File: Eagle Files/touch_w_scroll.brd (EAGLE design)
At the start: 14 x 73 mm, 3 parts

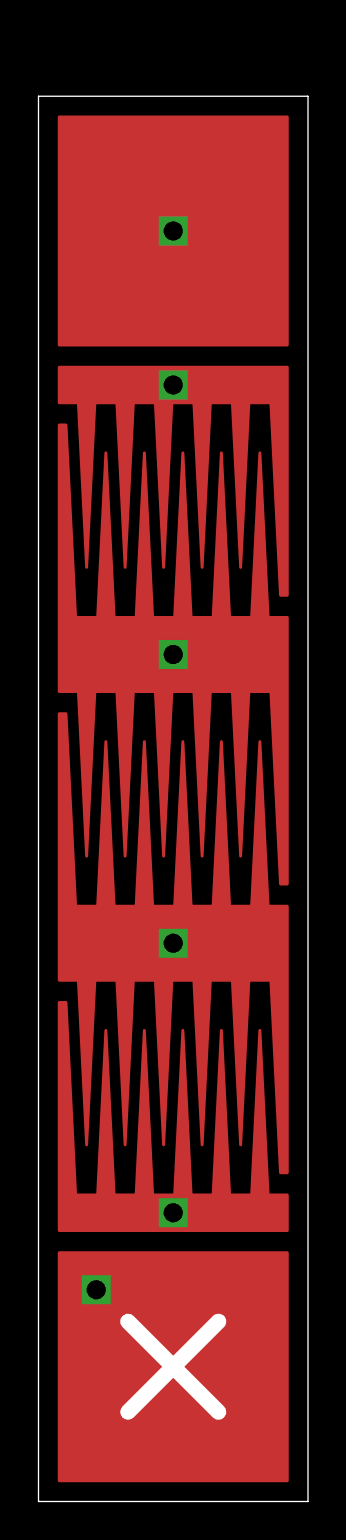
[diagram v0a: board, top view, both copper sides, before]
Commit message: maybe final touch board
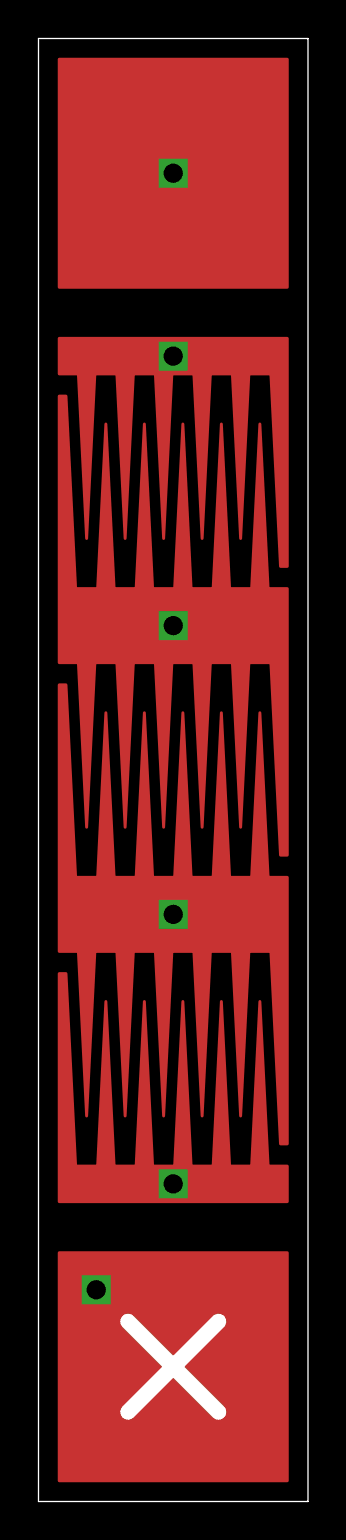
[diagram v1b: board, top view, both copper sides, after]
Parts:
- moved U$2 3.00 mm to (1.00, 75.0)
- moved U$1 1.50 mm to (13.0, 60.5)
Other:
- board size 14 x 73 mm -> 14 x 76 mm
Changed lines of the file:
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@@
 <layer number="44" name="Drills" color="7" fill="1" visible="no" active="yes"/>
 <layer number="45" name="Holes" color="7" fill="1" visible="no" active="yes"/>
-<layer number="46" name="Milling" color="3" fill="1" visible="no" active="yes"/>
+<layer number="46" name="Milling" color="3" fill="1" visible="yes" active="yes"/>
 <layer number="47" name="Measures" color="7" fill="1" visible="no" active="yes"/>
 <layer number="48" name="Document" color="7" fill="1" visible="yes" active="yes"/>
@@
 <plain>
 <wire x1="0" y1="0" x2="14" y2="0" width="0" layer="20"/>
-<wire x1="14" y1="0" x2="14" y2="73" width="0" layer="20"/>
-<wire x1="14" y1="73" x2="0" y2="73" width="0" layer="20"/>
-<wire x1="0" y1="73" x2="0" y2="0" width="0" layer="20"/>
-<wire x1="4.65" y1="9.35" x2="9.35" y2="4.65" width="0.8128" layer="20"/>
-<wire x1="4.65" y1="4.65" x2="9.35" y2="9.35" width="0.8128" layer="20"/>
+<wire x1="14" y1="0" x2="14" y2="76" width="0" layer="20"/>
+<wire x1="14" y1="76" x2="0" y2="76" width="0" layer="20"/>
+<wire x1="0" y1="76" x2="0" y2="0" width="0" layer="20"/>
 </plain>
 <attributes>
@@
 </autorouter>
 <elements>
-<element name="U$1" library="Cap Touch Pads" library_urn="urn:adsk.eagle:library:35100943" package="SLIDE" package3d_urn="urn:adsk.eagle:package:35100947/4" value="SLIDE_PAD" x="13" y="59" smashed="yes" rot="R270"/>
-<element name="U$2" library="Cap Touch Pads" library_urn="urn:adsk.eagle:library:35100943" package="12X12_PAD" package3d_urn="urn:adsk.eagle:package:35100948/2" value="12X12_PAD" x="1" y="72" smashed="yes"/>
-<element name="U$4" library="Cap Touch Pads" library_urn="urn:adsk.eagle:library:35100943" package="12X12_PAD_LED" package3d_urn="urn:adsk.eagle:package:35129608/1" value="12X12_PADLED" x="1" y="13" smashed="yes"/>
+<element name="U$1" library="Cap Touch Pads" library_urn="urn:adsk.eagle:library:35100943" package="SLIDE" package3d_urn="urn:adsk.eagle:package:35100947/4" value="SLIDE_PAD" x="13" y="60.5" smashed="yes" rot="R270"/>
+<element name="U$2" library="Cap Touch Pads" library_urn="urn:adsk.eagle:library:35100943" package="12X12_PAD" package3d_urn="urn:adsk.eagle:package:35100948/2" value="12X12_PAD" x="1" y="75" smashed="yes"/>
+<element name="U$4" library="Cap Touch Pads" library_urn="urn:adsk.eagle:library:35100943" package="12X12_PAD_LED" package3d_urn="urn:adsk.eagle:package:35129608/3" value="12X12_PADLED" x="1" y="13" smashed="yes"/>
 </elements>
 <signals>
@@
 <mfgpreviewcolor name="substratecolor" color="0xFF786E46"/>
 </mfgpreviewcolors>
+<errors>
+</errors>
 </board>
 </drawing>
